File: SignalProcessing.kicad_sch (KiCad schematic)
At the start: 31 parts, among them J5 Header_100mil_1x06, J6 Header_100mil_1x06, U14 ADS131M04IPWR, U15 AD9833BRMZ-REEL7, U16 AD826

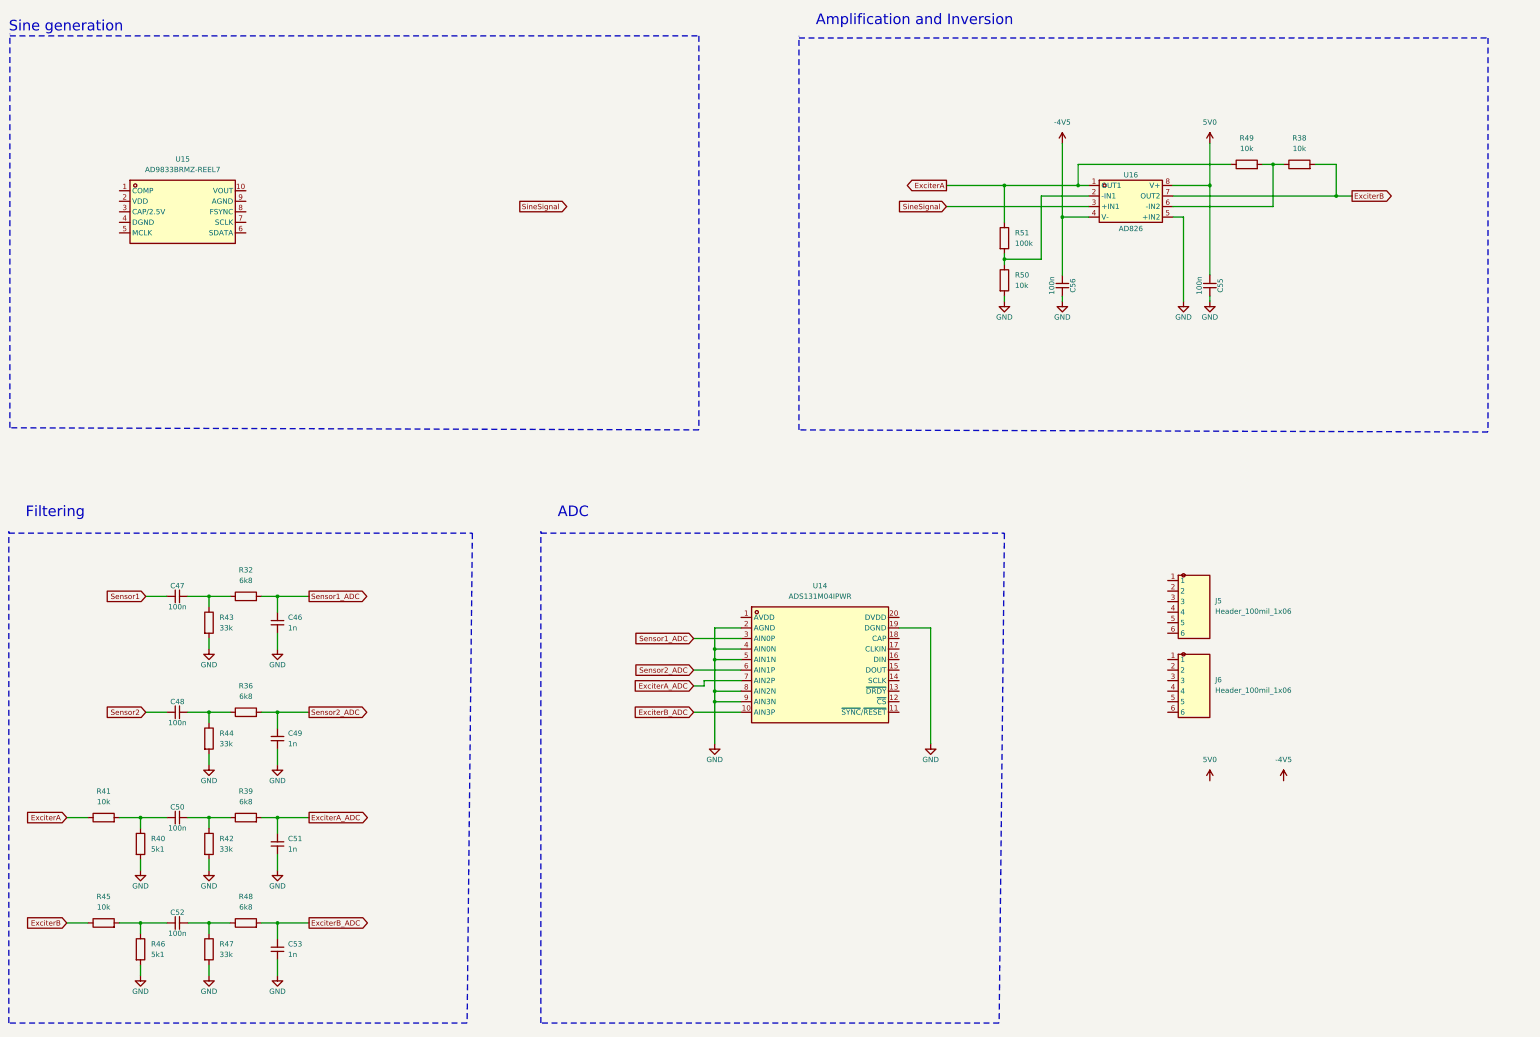
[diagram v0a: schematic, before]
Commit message: Schematic and component placement semi-final. Routing pending
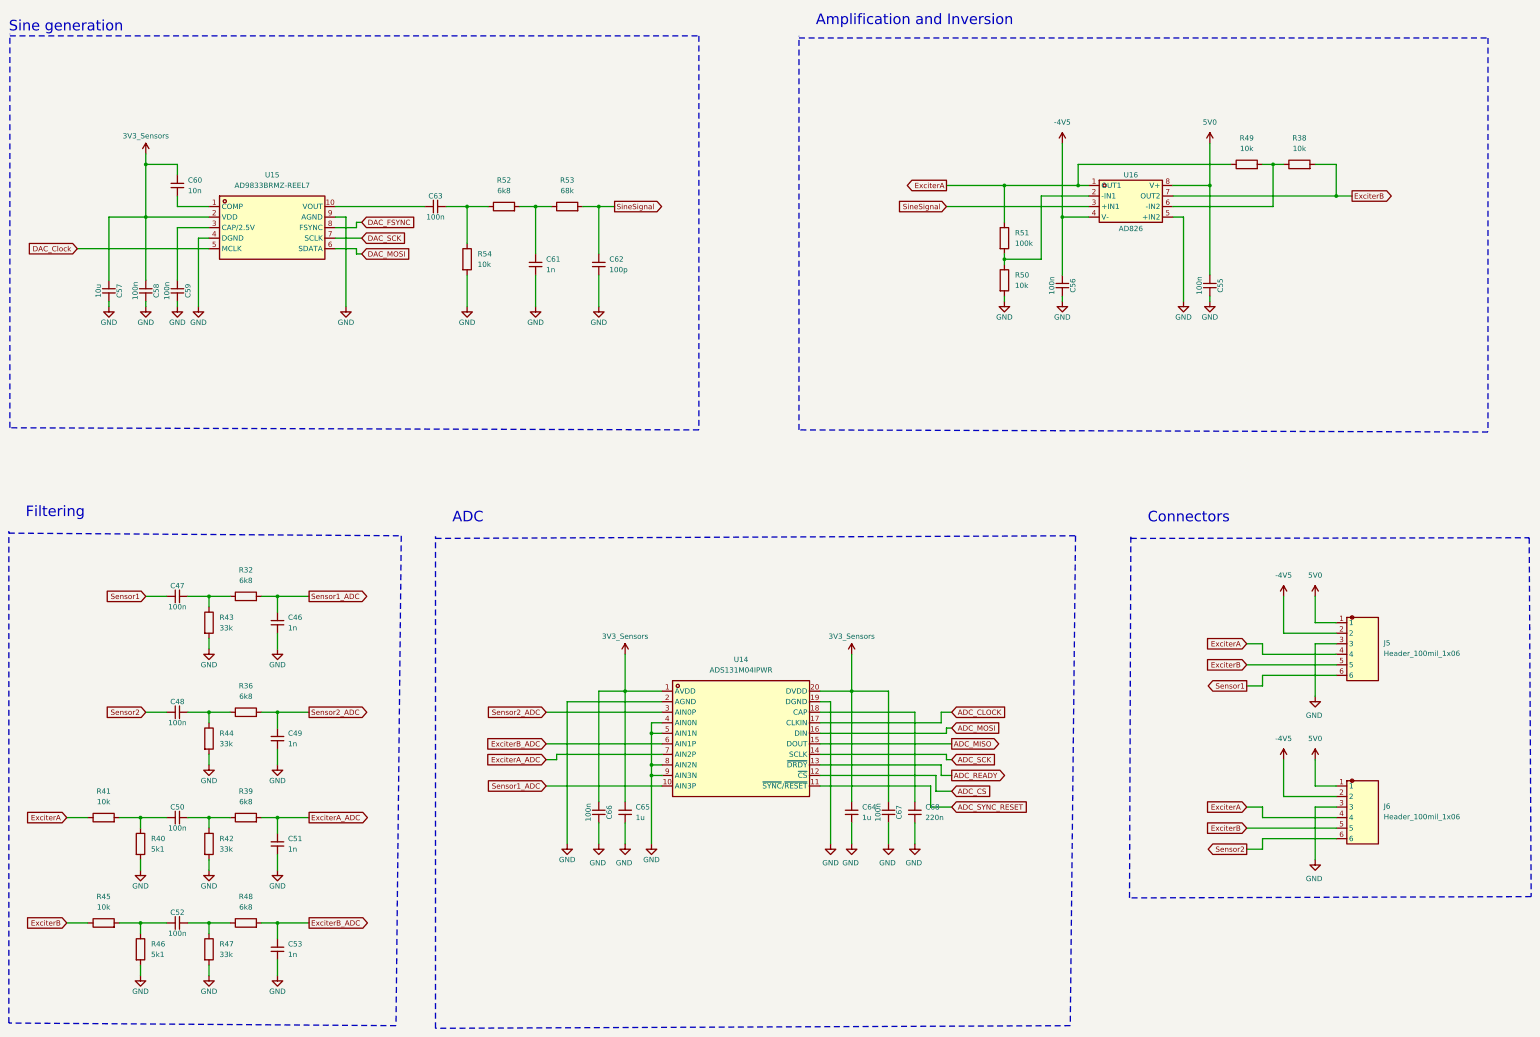
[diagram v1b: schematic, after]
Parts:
- added C57: 10u, sldrnrd:C_1206, symbol sldrnrd:Capacitor/C1206_10u
- added C58, C59, C63, C66, C67: 100n, sldrnrd:C_0603, symbol sldrnrd:Capacitor/C0603_100n
- added C60: 10n, sldrnrd:C_0603, symbol sldrnrd:Capacitor/C0603_10n
- added C61: 1n, sldrnrd:C_0603, symbol sldrnrd:Capacitor/C0603_1n
- added C62: 100p, sldrnrd:C_0603, symbol sldrnrd:Capacitor/C0603_100p
- added C64, C65: 1u, sldrnrd:C_0603, symbol sldrnrd:Capacitor/C0603_1u
- added C68: 220n, sldrnrd:C_0603, symbol sldrnrd:Capacitor/C0603_220n
- added R52: 6k8, sldrnrd:R_0603, symbol sldrnrd:Resistor/R0603_6k8
- added R53: 68k, sldrnrd:R_0603, symbol sldrnrd:Resistor/R0603_68k
- added R54: 10k, sldrnrd:R_0603, symbol sldrnrd:Resistor/R0603_10k
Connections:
- net -4V5: now also J5.2, J6.2
- net 5V0: now also J5.1, J6.1
- net ExciterA: now also J5.4, J6.4
- net ExciterB: now also J5.5, J6.5
- net ExciterB_ADC: now also U14.6 (AIN1P); no longer U14.10 (AIN3P)
- net GND: now also J5.3, J6.3, U15.4 (DGND), U15.9 (AGND), C57.2, C58.2, C59.2, C61.2, C62.2, C64.2, C65.2, C66.2, C67.2, C68.2, R54.2
- net Sensor1: now also J5.6
- net Sensor1_ADC: now also U14.10 (AIN3P); no longer U14.3 (AIN0P)
- net Sensor2: now also J6.6
- net Sensor2_ADC: now also U14.3 (AIN0P); no longer U14.6 (AIN1P)
- net SineSignal: now also C62.1, R53.2
- net at U15.1 (COMP): now also C60.2
- net at U15.10 (VOUT): now also C63.1
- net 3V3_Sensors: now reaches U15.2 (VDD)
- net 3V3_Sensors: now also U14.1 (AVDD), U14.20 (DVDD), C57.1, C58.1, C60.1, C64.1, C65.1, C66.1, C67.1
- net at U15.3 (CAP/2.5V): now also C59.1
- net DAC_Clock: now reaches U15.5 (MCLK)
- net DAC_MOSI: now reaches U15.6 (SDATA)
- net DAC_SCK: now reaches U15.7 (SCLK)
- net DAC_FSYNC: now reaches U15.8 (FSYNC)
- net ADC_SYNC_RESET: now reaches U14.11 (~{SYNC}/~{RESET})
- net ADC_CS: now reaches U14.12 (~{CS})
- net ADC_READY: now reaches U14.13 (~{DRDY})
- net ADC_SCK: now reaches U14.14 (SCLK)
- net ADC_MISO: now reaches U14.15 (DOUT)
- net ADC_MOSI: now reaches U14.16 (DIN)
- net ADC_CLOCK: now reaches U14.17 (CLKIN)
- net at U14.18 (CAP): now also C68.1
- new net: C63.2, R52.1, R54.1
- new net: C61.1, R52.2, R53.1
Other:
- note added: "Connectors"
- moved on the sheet: J5, U14, U15
